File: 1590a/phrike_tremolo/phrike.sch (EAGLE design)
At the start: 37 parts, among them Q1 2N5457, Q2 2N3904, Q3 2N5457, Q4 2N5088

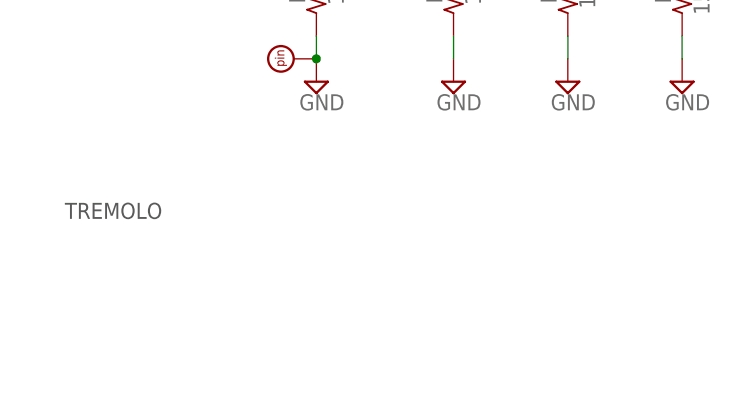
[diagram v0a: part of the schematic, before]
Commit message: finished chorus and tremolo baords; other tweaks & polish
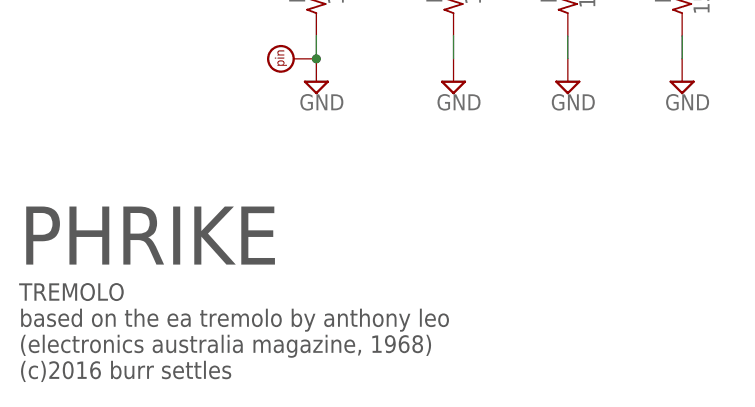
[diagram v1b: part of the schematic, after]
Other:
- note added: "PHRIKE"
- note added: "TREMOLO based on the ea tremolo by anthony leo (electronics australia magazine, 1968) (c)2016 burr settles"
- note removed: "TREMOLO"
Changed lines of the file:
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@@
 <sheet>
 <plain>
-<text x="7.62" y="20.32" size="1.778" layer="97">TREMOLO</text>
+<text x="2.54" y="15.24" size="6.4516" layer="97">PHRIKE</text>
+<text x="2.54" y="2.54" size="1.9304" layer="97">TREMOLO
+based on the ea tremolo by anthony leo
+(electronics australia magazine, 1968)
+(c)2016 burr settles</text>
 </plain>
 <instances>
@@
 </schematic>
 </drawing>
+<compatibility>
+<note version="6.3" minversion="6.2.2" severity="warning">
+Since Version 6.2.2 text objects can contain more than one line,
+which will not be processed correctly with this version.
+</note>
+</compatibility>
 </eagle>
